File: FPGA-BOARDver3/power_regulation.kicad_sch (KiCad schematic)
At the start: 29 parts, among them J1 PJ-102AH, J2 Conn_01x01_Pin, J3 Conn_01x03_Pin, Q7 DMG2305UX-13, U14 TLV62130RGTT, U15 LP5907MFX-3.3, U16 REF3012

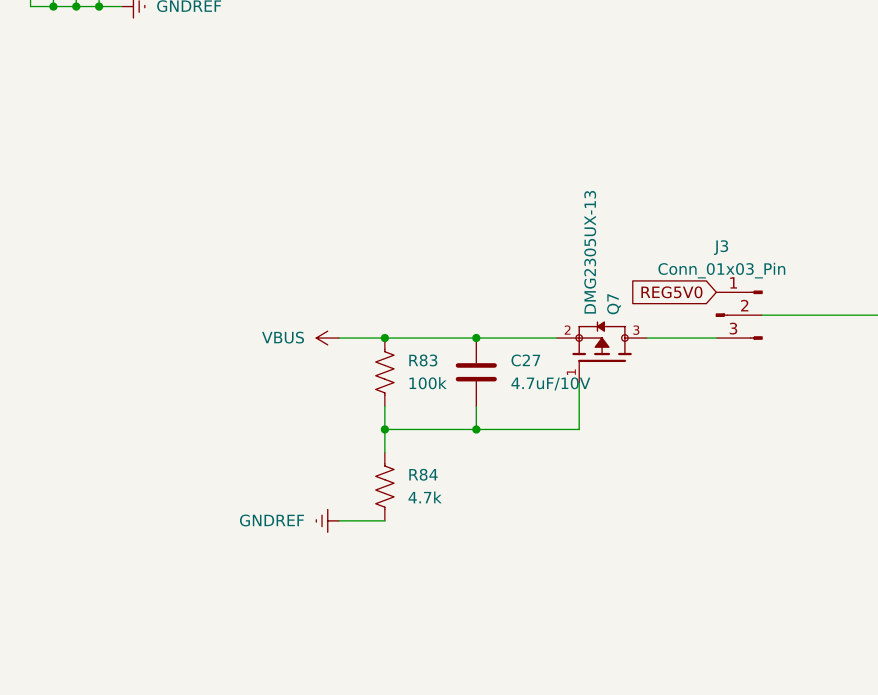
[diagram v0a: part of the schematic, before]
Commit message: update
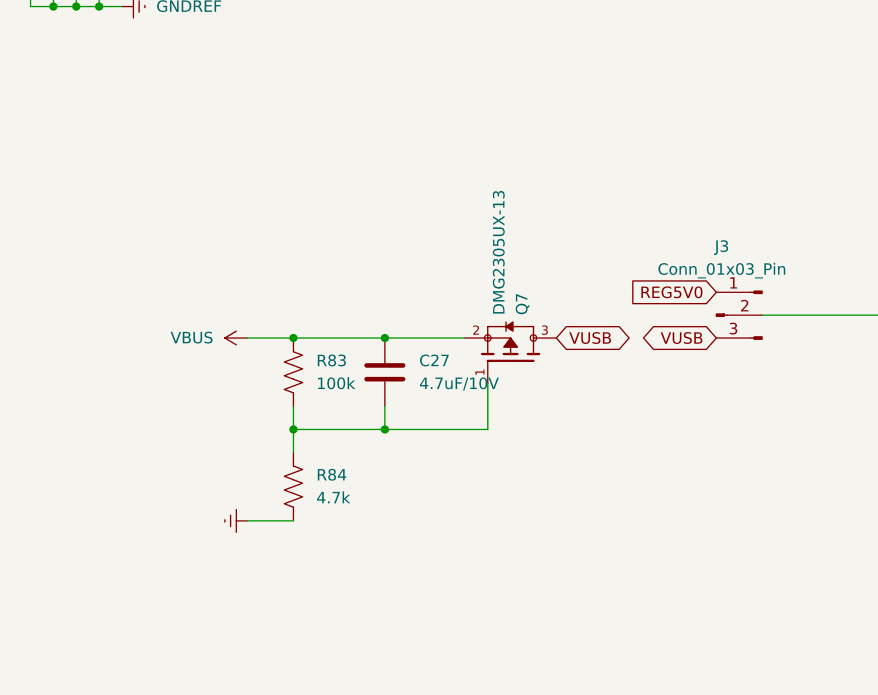
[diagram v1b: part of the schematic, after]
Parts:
- J2: footprint Connector_PinHeader_2.54mm:PinHeader_1x01_P2.54mm_Vertical -> footprints:PinHeader_1x01_P2.54mm_Vertical
- J3: footprint Connector_PinHeader_2.54mm:PinHeader_1x03_P2.54mm_Vertical -> footprints:PinHeader_1x03_P2.54mm_Vertical
- U15: footprint Package_TO_SOT_SMD:SOT-23-5 -> footprints:SOT-23-5
- U16: footprint Package_TO_SOT_SMD:SOT-23 -> footprints:SOT-23
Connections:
- net VUSB: now reaches J3.3 (Pin_3), Q7.3
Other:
- moved on the sheet: C27, Q7, R83, R84
